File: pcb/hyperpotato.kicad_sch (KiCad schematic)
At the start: 68 parts, among them J1 HRO_TYPE-C-31-M-14, J2 ELV1411A, J3 Conn_01x04_Socket, J4 Battery, Q1 AO3401A, Q2 2N7002, Q3 AO3401A, SW1 RST, SW10 SW_Push_45deg, SW11 SW_Push_45deg, SW12 SW_Push_45deg, SW13 SW_Push_45deg, SW14 SW_Push_45deg, SW15 PWR, SW2 SW_Push_45deg, SW3 SW_Push_45deg, SW4 SW_Push_45deg, SW5 SW_Push_45deg, SW6 SW_Push_45deg, SW7 SW_Push_45deg, SW8 SW_Push_45deg, SW9 SW_Push_45deg, U1 nRF52840_E73-2G4M08S1C, U2 DRV2605LDGS, U3 SRV05-4, U4 BQ24075, U5 SK8707-01, U6 SK8707-01-SENSOR, U7 MAX17048, Y1 32.768 KHz

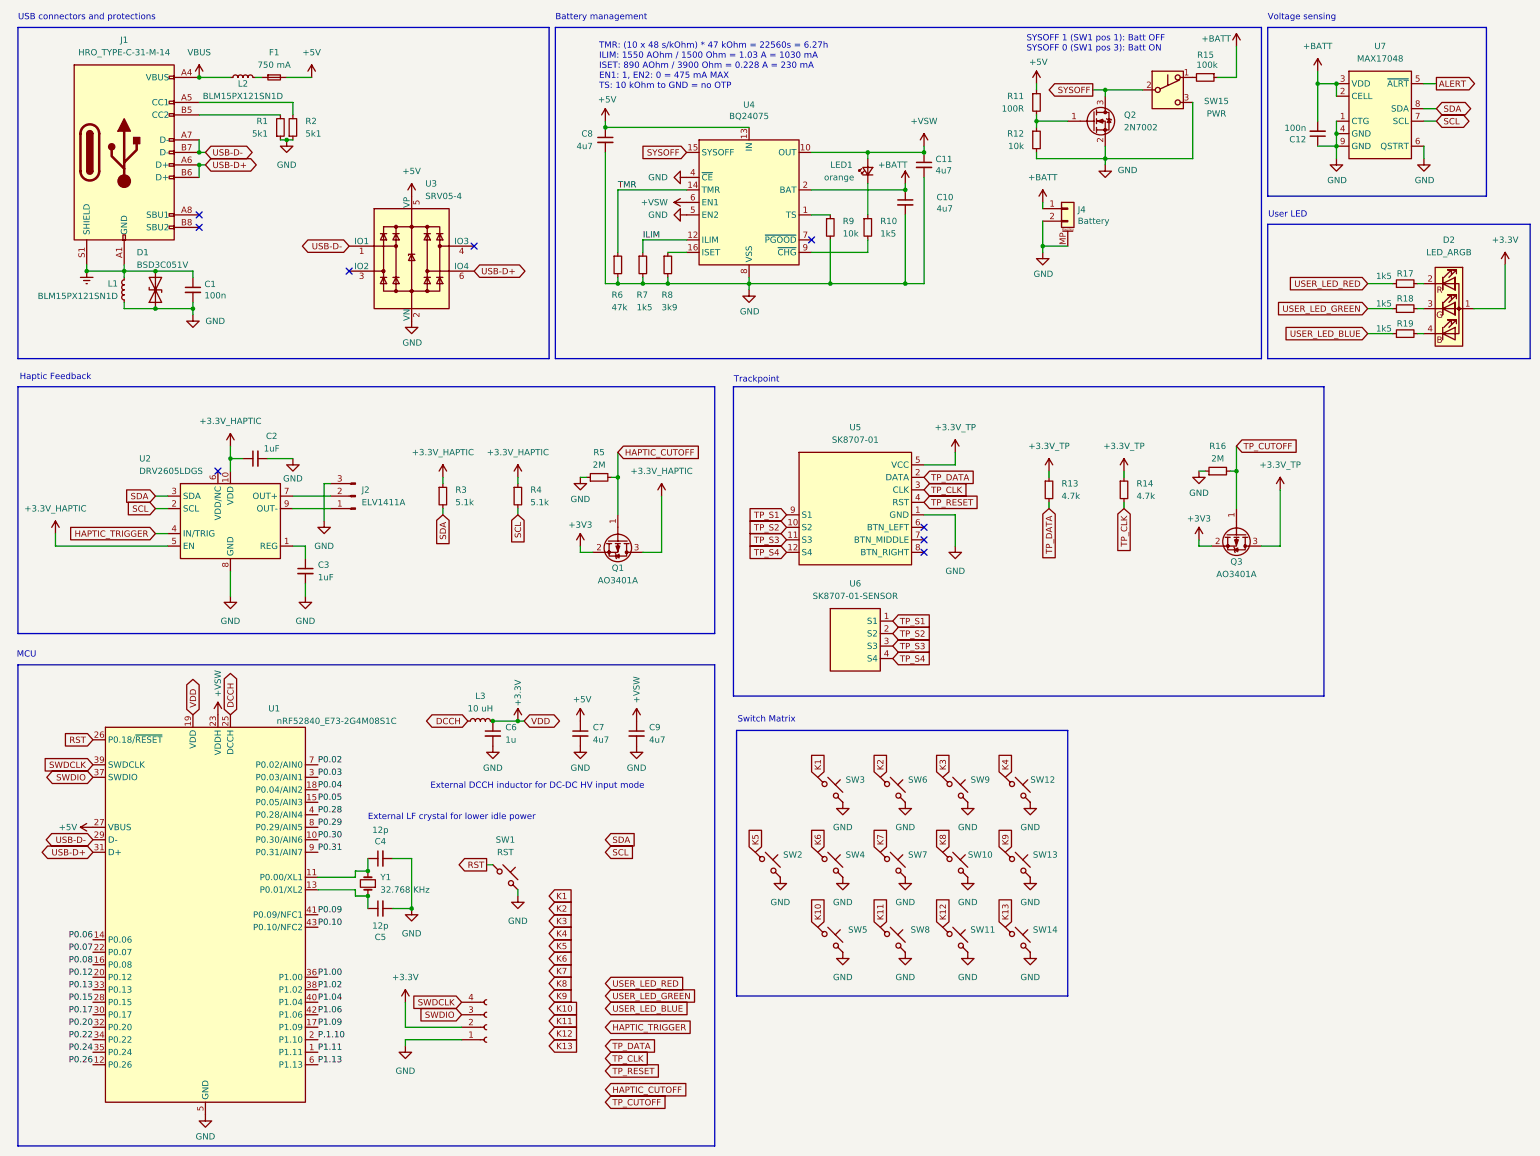
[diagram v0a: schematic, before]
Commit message: wip
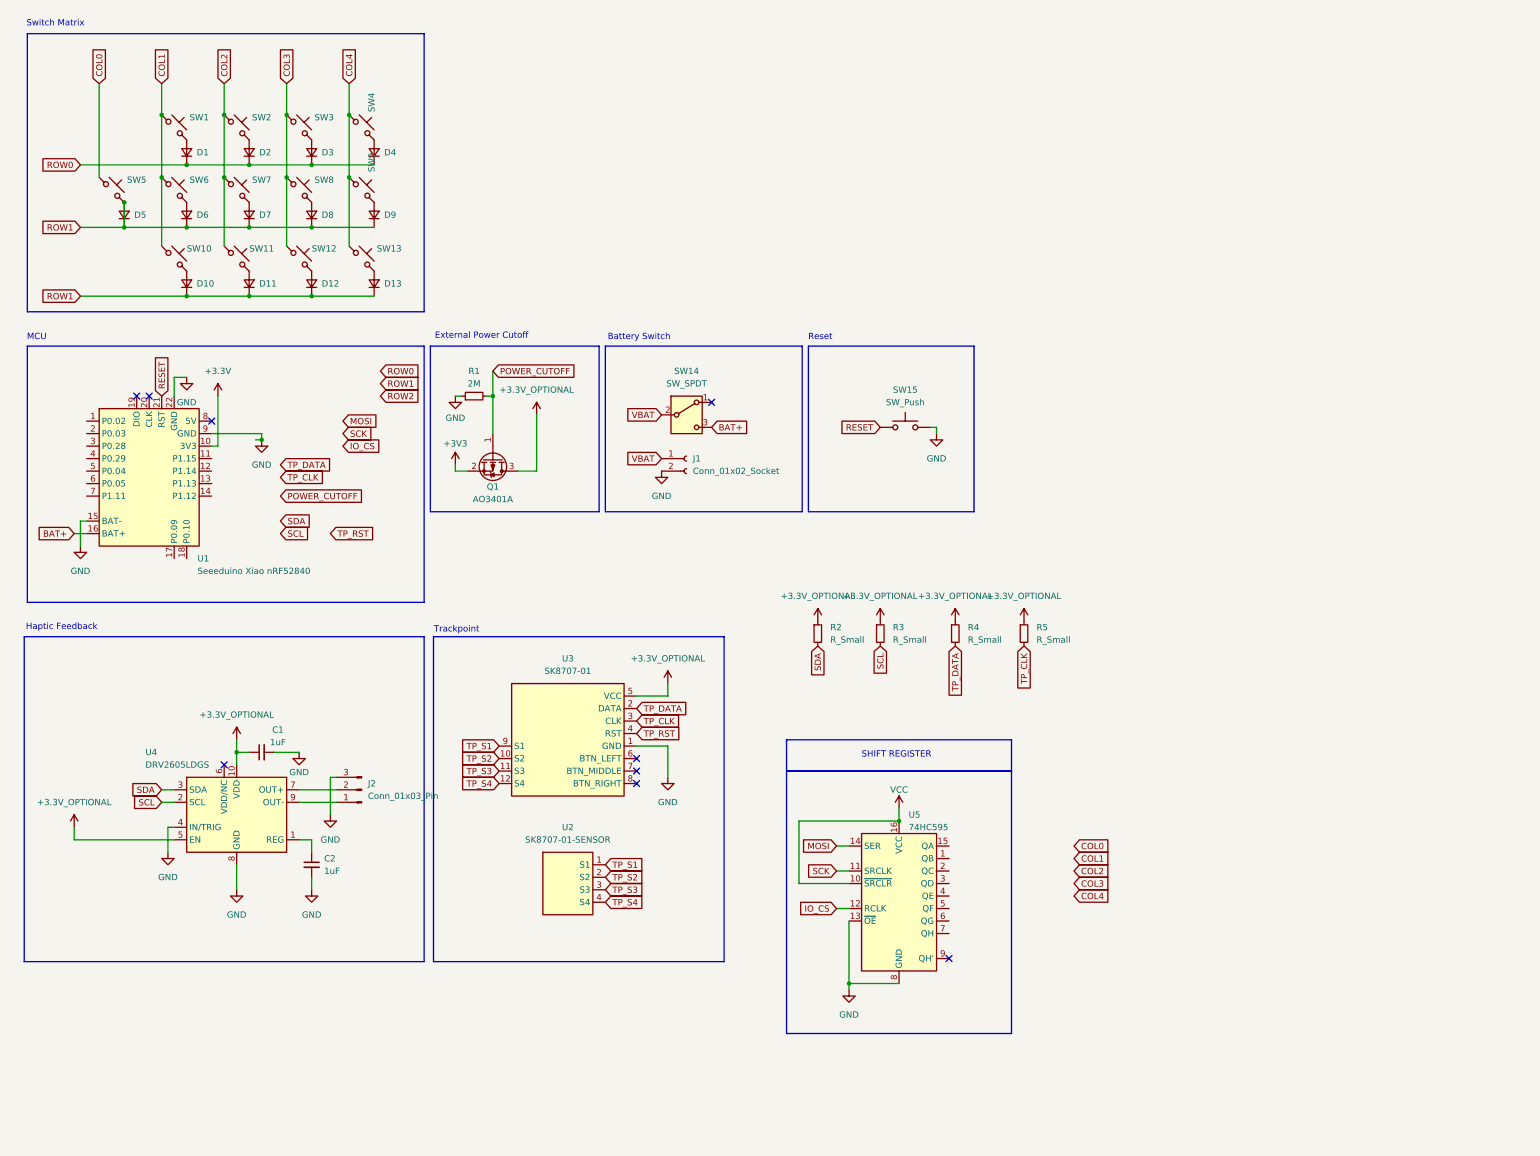
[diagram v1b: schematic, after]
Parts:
- removed C1, C12: 100n, ssbb_parts:C_0603_1608Metric_reversible, symbol Device:C_Small
- removed C10, C11, C7, C8, C9: 4u7, ssbb_parts:C_0603_1608Metric_reversible, symbol Device:C_Small
- removed C4, C5: 12p, ssbb_parts:C_0603_1608Metric_reversible, symbol Device:C_Small
- removed C6: 1u, ssbb_parts:C_0603_1608Metric_reversible, symbol Device:C_Small
- removed D1: BSD3C051V, ssbb_parts:D_SOD-323_reversible, symbol Device:D_TVS
- removed D2: LED_ARGB, symbol Device:LED_ARGB
- removed F1: 750 mA, ssbb_parts:Fuse_0603_1608Metric_reversible, symbol Device:Fuse_Small
- removed J1: HRO_TYPE-C-31-M-14, ssbb_parts:USB_C_Receptacle_HRO_TYPE-C-31-M-12_reversible, symbol Connector:USB_C_Receptacle_USB2.0
- removed J3: Conn_01x04_Socket, Connector_PinSocket_2.54mm:PinSocket_1x04_P2.54mm_Vertical, symbol Connector:Conn_01x04_Socket
- removed J4: Battery, ssbb_parts:Molex_Pico-EZmate_78171-0002_1x02-1MP_P1.20mm_Vertical_reversible, symbol Connector_Generic_MountingPin:Conn_01x02_MountingPin
- removed L1, L2: BLM15PX121SN1D, ssbb_parts:L_0603_1608Metric_reversible, symbol Device:L_Small
- removed L3: 10 uH, ssbb_parts:L_0603_1608Metric_reversible, symbol Device:L_Small
- removed LED1: orange, ssbb_parts:LED_0603_1608Metric_reversible, symbol Device:LED_Small
- removed Q2: 2N7002, ssbb_parts:SOT-23_reversible, symbol Transistor_FET:2N7002
- removed Q3: AO3401A, ssbb_parts:SOT-23_reversible, symbol Transistor_FET:AO3401A
- removed R1: 5k1, ssbb_parts:R_0603_1608Metric_reversible, symbol Device:R_Small
- removed R10, R17, R18, R19, R7: 1k5, ssbb_parts:R_0603_1608Metric_reversible, symbol Device:R_Small
- removed R11: 100R, ssbb_parts:R_0603_1608Metric_reversible, symbol Device:R_Small
- removed R12, R9: 10k, ssbb_parts:R_0603_1608Metric_reversible, symbol Device:R_Small
- removed R13, R14: 4.7k, ssbb_parts:R_0603_1608Metric_reversible, symbol Device:R_Small
- removed R15: 100k, ssbb_parts:R_0603_1608Metric_reversible, symbol Device:R_Small
- removed R16: 2M, ssbb_parts:R_0603_1608Metric_reversible, symbol Device:R_Small
- removed R6: 47k, ssbb_parts:R_0603_1608Metric_reversible, symbol Device:R_Small
- removed R8: 3k9, ssbb_parts:R_0603_1608Metric_reversible, symbol Device:R_Small
- removed SW1: RST, ssbb_parts:Panasonic_EVQPUL_EVQPUC_reversible, symbol Switch:SW_Push_45deg
- removed SW14: SW_Push_45deg, ssbb_parts:SW_choc_v1_reversible_1.5u, symbol Switch:SW_Push_45deg
- removed SW15: PWR, ssbb_parts:SW_SPDT_PCM12_reversible, symbol Switch:SW_Push_SPDT
- removed SW2, SW8: SW_Push_45deg, ssbb_parts:SW_choc_v1_reversible_1u, symbol Switch:SW_Push_45deg
- removed U1: nRF52840_E73-2G4M08S1C, ssbb_parts:nRF52840_E73-2G4M08S1C_reversible, symbol PCM_marbastlib-various:nRF52840_E73-2G4M08S1C
- removed U3: SRV05-4, ssbb_parts:SOT-23-6_reversible, symbol Power_Protection:SRV05-4
- removed U4: BQ24075, ssbb_parts:VQFN-16-1EP_3x3mm_P0.5mm_EP1.6x1.6mm_reversible, symbol Battery_Management:BQ24075RGT
- removed U5: SK8707-01, symbol ssbb_parts:Sprintek_SK8707–01
- removed U6: SK8707-01-SENSOR, ssbb_parts:Sprintek_SK8707-01_Sensor, symbol ssbb_parts:Sprintek_SK8707-01_Sensor
- removed U7: MAX17048, ssbb_parts:DFN-8-1EP_2x2mm_P0.5mm_EP0.6x1.2mm_reversible, symbol marbastlib-various:MAX17048
- removed Y1: 32.768 KHz, ssbb_parts:Crystal_SMD_2012-2Pin_2.0x1.2mm_reversible, symbol Device:Crystal_Small
- added D1, D10, D11, D12, D13, D2, D3, D4, D5, D6, D7, D8, D9: D_Small, ssbb_parts:D_0603_1608Metric_reversible, symbol Device:D_Small
- added J1: Conn_01x02_Socket, ssbb_parts:Molex_Pico-EZmate_78171-0002_1x02-1MP_P1.20mm_Vertical_reversible, symbol Connector:Conn_01x02_Socket
- added R5: R_Small, ssbb_parts:R_0603_1608Metric_reversible, symbol Device:R_Small
- added SW10, SW12: SW_Push_45deg, ssbb_parts:SW_choc_v1_reversible_1u, symbol Switch:SW_Push_45deg
- added SW13: SW_Push_45deg, ssbb_parts:SW_choc_v1_reversible_1.5u, symbol Switch:SW_Push_45deg
- added SW14: SW_SPDT, ssbb_parts:SW_SPDT_PCM12_reversible, symbol Switch:SW_SPDT
- added SW15: SW_Push, ssbb_parts:Panasonic_EVQPUL_EVQPUC_reversible, symbol Switch:SW_Push
- added U1: Seeeduino Xiao nRF52840, ssbb_parts:Xiao_nRF52840_AC_Reflow_reversible, symbol PCM_marbastlib-promicroish:Seeeduino_Xiao_nRF52840
- added U2: SK8707-01-SENSOR, ssbb_parts:Sprintek_SK8707-01_Sensor, symbol ssbb_parts:Sprintek_SK8707-01_Sensor
- added U3: SK8707-01, symbol ssbb_parts:Sprintek_SK8707–01
- added U5: 74HC595, ssbb_parts:TSSOP-16_4.4x5mm_P0.65mm_reversible, symbol 74xx:74HC595
- J2: value ELV1411A -> Conn_01x03_Pin
- R2: value 5k1 -> R_Small
- R3, R4: value 5.1k -> R_Small
- renumbered C2 to C1, C3 to C2, R5 to R1, SW3 to SW1, SW6 to SW2, SW9 to SW3, SW12 to SW4, SW4 to SW6, SW10 to SW8, SW13 to SW9, U2 to U4
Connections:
- net HAPTIC_TRIGGER is gone; now on net GND: U4.4 (IN/TRIG)
- net K2 is gone; now on net COL2: SW2.1
- net K6 is gone; now on net COL1: SW6.1
- net K7 is gone; now on net COL2: SW7.1
- net K8 is gone; now on net COL3: SW8.1
- net +3.3V: now also U1.10 (3V3)
- net GND: now also J1.2 (Pin_2), SW15.2, U1.15 (BAT-), U1.22 (GND), U1.9 (GND), U3.1 (GND), U5.13 (~{OE}), U5.8 (GND); no longer R2.1, SW1.2, SW11.2, SW2.2, SW3.2, SW4.2, SW5.2, SW6.2, SW7.2, SW8.2, SW9.2
- net SCL: now also R3.2; no longer R4.2
- net SDA: now also R2.2; no longer R3.2
- net TP_CLK: now also R5.2, U3.3 (CLK)
- net TP_DATA: now also R4.2, U3.2 (DATA)
- net TP_S1: now also U2.1 (S1), U3.9 (S1)
- net TP_S2: now also U2.2 (S2), U3.10 (S2)
- net TP_S3: now also U2.3 (S3), U3.11 (S3)
- net TP_S4: now also U2.4 (S4), U3.12 (S4)
- net +3.3V_HAPTIC renamed +3.3V_OPTIONAL
- net +3.3V_OPTIONAL: now also R2.1, R5.1, U3.5 (VCC)
- net HAPTIC_CUTOFF renamed POWER_CUTOFF
- net K1 renamed COL1
- net COL1: now also SW10.1
- net K10 renamed COL0
- net K12 renamed COL2
- net K3 renamed COL3
- net COL3: now also SW12.1
- net K4: no longer names the net of SW4.1
- net K4: now also D4.2 (A)
- net K9: no longer names the net of SW9.1
- net K9: now also D9.2 (A)
- new net: D8.2 (A), SW8.2
- new net: D13.2 (A), SW13.2
- new net: D10.2 (A), SW10.2
- new net: D1.2 (A), SW1.2
- new net: D12.2 (A), SW12.2
- new net: D3.2 (A), SW3.2
- new net: D2.2 (A), SW2.2
- new net: D7.2 (A), SW7.2
- new net: D6.2 (A), SW6.2
- new net: D11.2 (A), SW11.2
- new net BAT+: SW14.3 (C), U1.16 (BAT+)
- new net COL4: SW13.1, SW4.2, SW9.2
- new net IO_CS: U5.12 (RCLK)
- new net MOSI: U5.14 (SER)
- new net RESET: SW15.1, U1.21 (RST)
- new net ROW0: D1.1 (K), D2.1 (K), D3.1 (K), D4.1 (K)
- new net ROW1: D10.1 (K), D11.1 (K), D12.1 (K), D13.1 (K), D5.1 (K), D5.2 (A), D6.1 (K), D7.1 (K), D8.1 (K), D9.1 (K), SW5.2
- new net SCK: U5.11 (SRCLK)
- new net TP_RST: U3.4 (RST)
- new net VBAT: J1.1 (Pin_1), SW14.2 (B)
- new net VCC: U5.10 (~{SRCLR}), U5.16 (VCC)
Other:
- note added: "Battery Switch"
- note added: "External Power Cutoff"
- note added: "Reset"
- note added: "SHIFT REGISTER"
- note removed: "Battery management"
- note removed: "External DCCH inductor for DC-DC HV input mode"
- note removed: "External LF crystal for lower idle power"
- note removed: "SYSOFF 1 (SW1 pos 1): Batt OFF SYSOFF 0 (SW1 pos 3): Batt ON"
- note removed: "TMR: (10 x 48 s/kOhm) * 47 kOhm = 22560s = 6.27h ILIM: 1550 AOhm / 1500 Ohm = 1.03 A = 1030 mA ISET: 890 AOhm / 3900 Ohm = 0.228 A = 230 mA EN1: 1, EN2: 0 = 475 mA MAX TS: 10 kOhm to GND = no OTP"
- note removed: "USB connectors and protections"
- note removed: "User LED"
- note removed: "Voltage sensing"
- moved on the sheet: C1, C2, Q1, R1, SW1, SW2, SW3, SW4, SW6, SW7, SW8, SW9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

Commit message: wip arrange
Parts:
- D1, D10, D11, D12, D13, D2, D3, D4, D5, D6, D7, D8, D9: footprint ssbb_parts:D_0603_1608Metric_reversible -> ssbb_parts:D_SOD-123_reversible
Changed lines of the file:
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@@
 			)
 		)
-		(property "Footprint" "ssbb_parts:D_0603_1608Metric_reversible"
+		(property "Footprint" "ssbb_parts:D_SOD-123_reversible"
 			(at 73.66 54.61 90)
 			(effects
@@
 			)
 		)
-		(property "Footprint" "ssbb_parts:D_0603_1608Metric_reversible"
+		(property "Footprint" "ssbb_parts:D_SOD-123_reversible"
 			(at 35.56 54.61 90)
 			(effects
@@
 			)
 		)
-		(property "Footprint" "ssbb_parts:D_0603_1608Metric_reversible"
+		(property "Footprint" "ssbb_parts:D_SOD-123_reversible"
 			(at 86.36 54.61 90)
 			(effects
@@
 			)
 		)
-		(property "Footprint" "ssbb_parts:D_0603_1608Metric_reversible"
+		(property "Footprint" "ssbb_parts:D_SOD-123_reversible"
 			(at 86.36 68.58 90)
 			(effects
@@
 			)
 		)
-		(property "Footprint" "ssbb_parts:D_0603_1608Metric_reversible"
+		(property "Footprint" "ssbb_parts:D_SOD-123_reversible"
 			(at 48.26 41.91 90)
 			(effects
@@
 			)
 		)
-		(property "Footprint" "ssbb_parts:D_0603_1608Metric_reversible"
+		(property "Footprint" "ssbb_parts:D_SOD-123_reversible"
 			(at 73.66 68.58 90)
 			(effects
@@
 			)
 		)
-		(property "Footprint" "ssbb_parts:D_0603_1608Metric_reversible"
+		(property "Footprint" "ssbb_parts:D_SOD-123_reversible"
 			(at 48.26 68.58 90)
 			(effects
@@
 			)
 		)
-		(property "Footprint" "ssbb_parts:D_0603_1608Metric_reversible"
+		(property "Footprint" "ssbb_parts:D_SOD-123_reversible"
 			(at 60.96 41.91 90)
 			(effects
@@
 			)
 		)
-		(property "Footprint" "ssbb_parts:D_0603_1608Metric_reversible"
+		(property "Footprint" "ssbb_parts:D_SOD-123_reversible"
 			(at 60.96 54.61 90)
 			(effects
@@
 			)
 		)
-		(property "Footprint" "ssbb_parts:D_0603_1608Metric_reversible"
+		(property "Footprint" "ssbb_parts:D_SOD-123_reversible"
 			(at 86.36 41.91 90)
 			(effects
@@
 			)
 		)
-		(property "Footprint" "ssbb_parts:D_0603_1608Metric_reversible"
+		(property "Footprint" "ssbb_parts:D_SOD-123_reversible"
 			(at 73.66 41.91 90)
 			(effects
@@
 			)
 		)
-		(property "Footprint" "ssbb_parts:D_0603_1608Metric_reversible"
+		(property "Footprint" "ssbb_parts:D_SOD-123_reversible"
 			(at 60.96 68.58 90)
 			(effects
@@
 			)
 		)
-		(property "Footprint" "ssbb_parts:D_0603_1608Metric_reversible"
+		(property "Footprint" "ssbb_parts:D_SOD-123_reversible"
 			(at 48.26 54.61 90)
 			(effects
